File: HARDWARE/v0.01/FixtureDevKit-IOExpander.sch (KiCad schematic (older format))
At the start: 58 parts

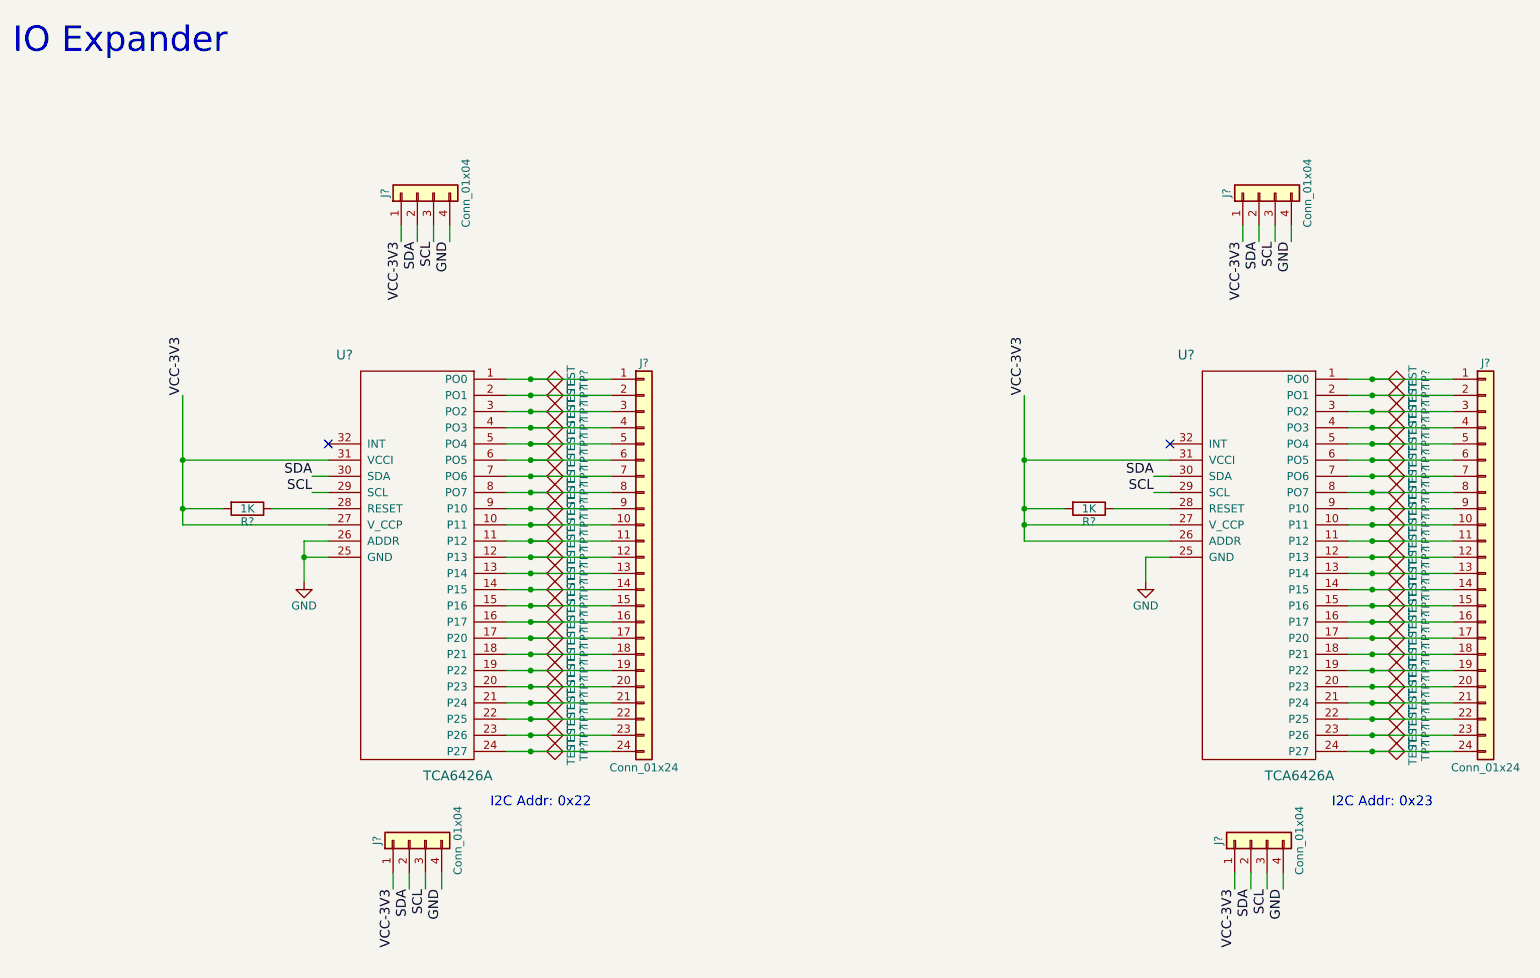
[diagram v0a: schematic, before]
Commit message: o boy
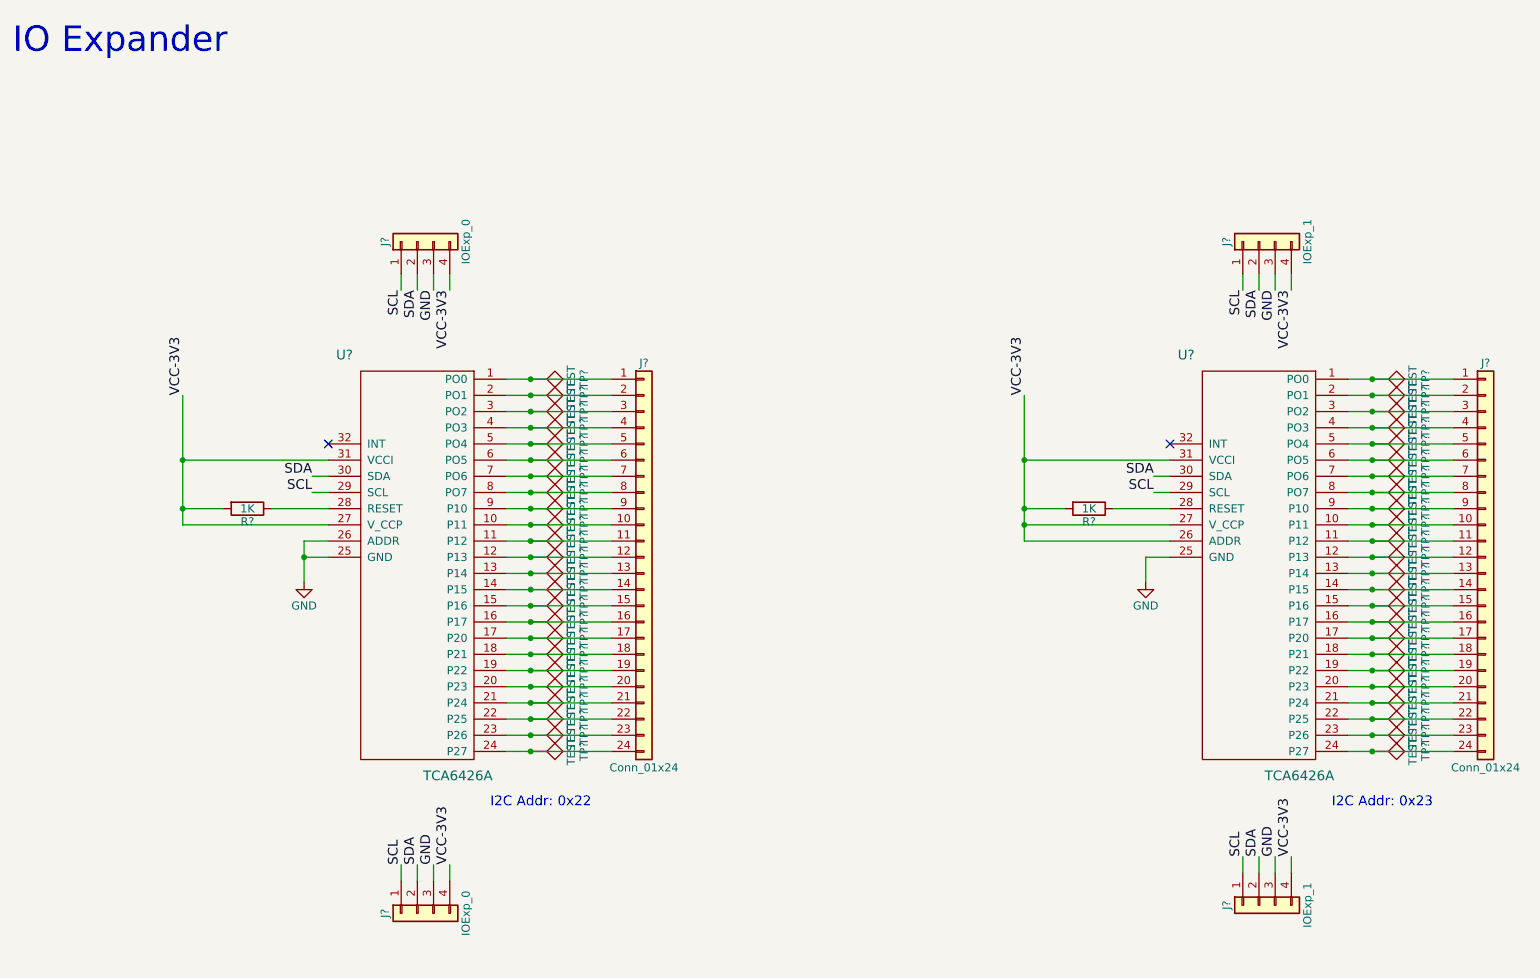
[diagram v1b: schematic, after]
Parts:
- removed J? (x3): Conn_01x04, symbol Conn_01x04
- added J?: IOExp_0, symbol Conn_01x04
- added J? (x2): IOExp_1, symbol Conn_01x04
- J?: value Conn_01x04 -> IOExp_0
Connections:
- net GND: now also J?.3 (Pin_3), J?.3 (Pin_3), J?.3 (Pin_3), J?.3 (Pin_3); no longer J?.4 (Pin_4)
- net SCL: now also J?.1 (Pin_1), J?.1 (Pin_1), J?.1 (Pin_1), J?.1 (Pin_1); no longer J?.3 (Pin_3)
- net SDA: now also J?.2 (Pin_2), J?.2 (Pin_2), J?.2 (Pin_2)
- net VCC-3V3: now also J?.4 (Pin_4), J?.4 (Pin_4), J?.4 (Pin_4), J?.4 (Pin_4); no longer J?.1 (Pin_1)
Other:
- moved on the sheet: J?
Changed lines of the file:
@@
 L Conn_01x04 J?
 U 1 1 59EFBDCF
-P 3250 1700
-F 0 "J?" H 3250 1900 50  0000 C CNN
-F 1 "Conn_01x04" H 3250 1400 50  0000 C CNN
-F 2 "" H 3250 1700 50  0001 C CNN
-F 3 "" H 3250 1700 50  0001 C CNN
-	1    3250 1700
+P 3250 2000
+F 0 "J?" H 3250 2200 50  0000 C CNN
+F 1 "IOExp_0" H 3250 1700 50  0000 C CNN
+F 2 "" H 3250 2000 50  0001 C CNN
+F 3 "" H 3250 2000 50  0001 C CNN
+	1    3250 2000
 	0    -1   -1   0
 $EndComp
-Text Label 3150 2000 3    60   ~ 0
+Text Label 3150 2300 3    60   ~ 0
+SCL
+Text Label 3250 2300 3    60   ~ 0
+SDA
+Text Label 3350 2300 3    60   ~ 0
+GND
+Text Label 3450 2300 3    60   ~ 0
 VCC-3V3
-Text Label 3250 2000 3    60   ~ 0
-SDA
-Text Label 3350 2000 3    60   ~ 0
-SCL
-Text Label 3450 2000 3    60   ~ 0
-GND
 Text Label 2600 3450 2    60   ~ 0
 SDA
@@
 	2600 3550 2700 3550
 Wire Wire Line
-	3450 2000 3450 1900
-Wire Wire Line
-	3350 1900 3350 2000
-Wire Wire Line
-	3250 2000 3250 1900
-Wire Wire Line
-	3150 1900 3150 2000
-$Comp
-L Conn_01x04 J?
-U 1 1 59EFCA72
-P 3200 5700
-F 0 "J?" H 3200 5900 50  0000 C CNN
-F 1 "Conn_01x04" H 3200 5400 50  0000 C CNN
-F 2 "" H 3200 5700 50  0001 C CNN
-F 3 "" H 3200 5700 50  0001 C CNN
-	1    3200 5700
-	0    -1   -1   0
-$EndComp
-Text Label 3100 6000 3    60   ~ 0
-VCC-3V3
-Text Label 3200 6000 3    60   ~ 0
-SDA
-Text Label 3300 6000 3    60   ~ 0
-SCL
-Text Label 3400 6000 3    60   ~ 0
-GND
-Wire Wire Line
-	3400 6000 3400 5900
-Wire Wire Line
-	3300 5900 3300 6000
-Wire Wire Line
-	3200 6000 3200 5900
-Wire Wire Line
-	3100 5900 3100 6000
+	3450 2300 3450 2200
+Wire Wire Line
+	3350 2200 3350 2300
+Wire Wire Line
+	3250 2300 3250 2200
+Wire Wire Line
+	3150 2200 3150 2300
 $Comp
 L TCA6426A U?
@@
 	7900 3350 7000 3350
 Connection ~ 7000 3350
-$Comp
-L Conn_01x04 J?
-U 1 1 59EFEA17
-P 8450 1700
-F 0 "J?" H 8450 1900 50  0000 C CNN
-F 1 "Conn_01x04" H 8450 1400 50  0000 C CNN
-F 2 "" H 8450 1700 50  0001 C CNN
-F 3 "" H 8450 1700 50  0001 C CNN
-	1    8450 1700
-	0    -1   -1   0
-$EndComp
-Text Label 8350 2000 3    60   ~ 0
-VCC-3V3
-Text Label 8450 2000 3    60   ~ 0
-SDA
-Text Label 8550 2000 3    60   ~ 0
-SCL
-Text Label 8650 2000 3    60   ~ 0
-GND
 Text Label 7800 3450 2    60   ~ 0
 SDA
@@
 Wire Wire Line
 	7800 3550 7900 3550
-Wire Wire Line
-	8650 2000 8650 1900
-Wire Wire Line
-	8550 1900 8550 2000
-Wire Wire Line
-	8450 2000 8450 1900
-Wire Wire Line
-	8350 1900 8350 2000
-$Comp
-L Conn_01x04 J?
-U 1 1 59EFEA29
-P 8400 5700
-F 0 "J?" H 8400 5900 50  0000 C CNN
-F 1 "Conn_01x04" H 8400 5400 50  0000 C CNN
-F 2 "" H 8400 5700 50  0001 C CNN
-F 3 "" H 8400 5700 50  0001 C CNN
-	1    8400 5700
-	0    -1   -1   0
-$EndComp
-Text Label 8300 6000 3    60   ~ 0
-VCC-3V3
-Text Label 8400 6000 3    60   ~ 0
-SDA
-Text Label 8500 6000 3    60   ~ 0
-SCL
-Text Label 8600 6000 3    60   ~ 0
-GND
-Wire Wire Line
-	8600 6000 8600 5900
-Wire Wire Line
-	8500 5900 8500 6000
-Wire Wire Line
-	8400 6000 8400 5900
-Wire Wire Line
-	8300 5900 8300 6000
 Text Notes 750  850  0    157  ~ 0
 IO Expander
@@
 Text Notes 8900 5500 0    61   ~ 0
 I2C Addr: 0x23\n
+$Comp
+L Conn_01x04 J?
+U 1 1 59EFECEB
+P 3250 6150
+F 0 "J?" H 3250 6350 50  0000 C CNN
+F 1 "IOExp_0" H 3250 5850 50  0000 C CNN
+F 2 "" H 3250 6150 50  0001 C CNN
+F 3 "" H 3250 6150 50  0001 C CNN
+	1    3250 6150
+	0    -1   1    0
+$EndComp
+Text Label 3150 5850 1    60   ~ 0
+SCL
+Text Label 3250 5850 1    60   ~ 0
+SDA
+Text Label 3350 5850 1    60   ~ 0
+GND
+Text Label 3450 5850 1    60   ~ 0
+VCC-3V3
+Wire Wire Line
+	3450 5850 3450 5950
+Wire Wire Line
+	3350 5950 3350 5850
+Wire Wire Line
+	3250 5850 3250 5950
+Wire Wire Line
+	3150 5950 3150 5850
+$Comp
+L Conn_01x04 J?
+U 1 1 59EFFD29
+P 8450 2000
+F 0 "J?" H 8450 2200 50  0000 C CNN
+F 1 "IOExp_1" H 8450 1700 50  0000 C CNN
+F 2 "" H 8450 2000 50  0001 C CNN
+F 3 "" H 8450 2000 50  0001 C CNN
+	1    8450 2000
+	0    -1   -1   0
+$EndComp
+Text Label 8350 2300 3    60   ~ 0
+SCL
+Text Label 8450 2300 3    60   ~ 0
+SDA
+Text Label 8550 2300 3    60   ~ 0
+GND
+Text Label 8650 2300 3    60   ~ 0
+VCC-3V3
+Wire Wire Line
+	8650 2300 8650 2200
+Wire Wire Line
+	8550 2200 8550 2300
+Wire Wire Line
+	8450 2300 8450 2200
+Wire Wire Line
+	8350 2200 8350 2300
+$Comp
+L Conn_01x04 J?
+U 1 1 59EFFE87
+P 8450 6100
+F 0 "J?" H 8450 6300 50  0000 C CNN
+F 1 "IOExp_1" H 8450 5800 50  0000 C CNN
+F 2 "" H 8450 6100 50  0001 C CNN
+F 3 "" H 8450 6100 50  0001 C CNN
+	1    8450 6100
+	0    -1   1    0
+$EndComp
+Text Label 8350 5800 1    60   ~ 0
+SCL
+Text Label 8450 5800 1    60   ~ 0
+SDA
+Text Label 8550 5800 1    60   ~ 0
+GND
+Text Label 8650 5800 1    60   ~ 0
+VCC-3V3
+Wire Wire Line
+	8650 5800 8650 5900
+Wire Wire Line
+	8550 5900 8550 5800
+Wire Wire Line
+	8450 5800 8450 5900
+Wire Wire Line
+	8350 5900 8350 5800
 $EndSCHEMATC
